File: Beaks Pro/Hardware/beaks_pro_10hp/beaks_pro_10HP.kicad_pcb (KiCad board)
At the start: 2 copper layers, 135.8 x 108.6 mm, 124 parts, among them J1 Pins_02x10_P2.54mm_TH, J11 out1, J12 out2, J13 Eurorack Power, J14 Pins_02x10_P2.54mm_TH, J2 Pins_02x10_P2.54mm_TH, J3 CV1, J4 CV2, J5 CV3, J6 CV4, J7 in1, J8 in2, J9 Pins_02x10_P2.54mm_TH, Q1 2N3904, Q2 2N3904, SW2 SW_Dual, SW3 SW_Mode, SW5 SW_ML6, SW6 SW_ML6, U1 TL072CP, U2 MCP6002-I-P, U3 TL072CP, U4 MCP6002-I-P, U5 TL074, U6 LM4040LP-10, U7 L78L05_TO92, U8 Bluepill, U9 TL072CP

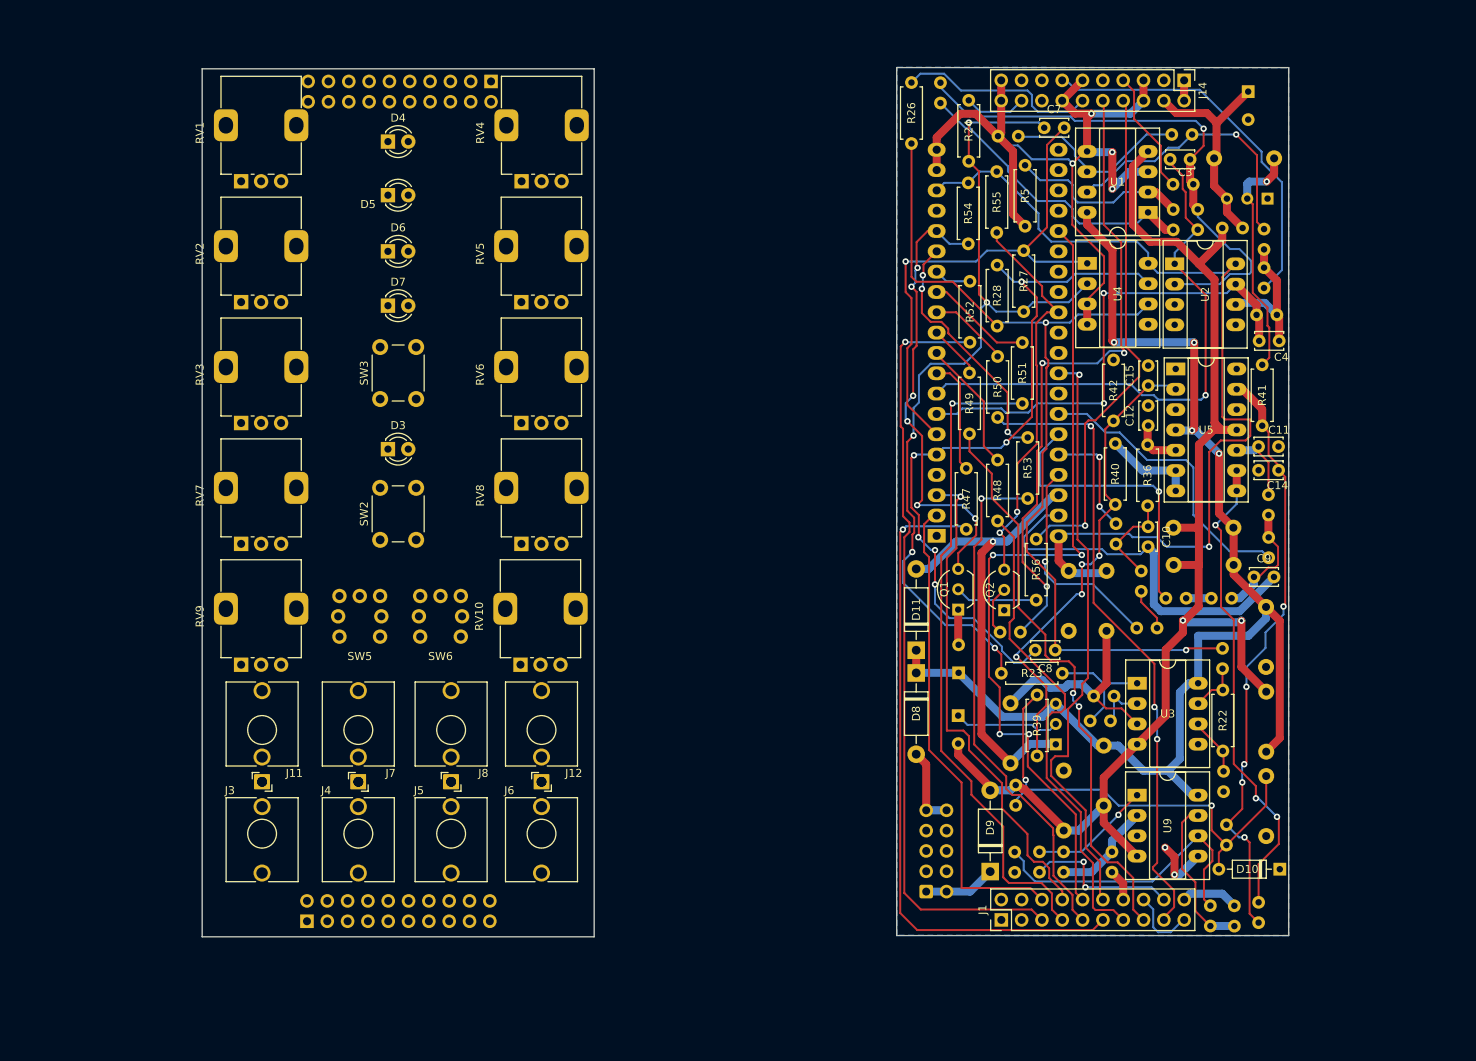
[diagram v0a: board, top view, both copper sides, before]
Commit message: V0.1 Alpha
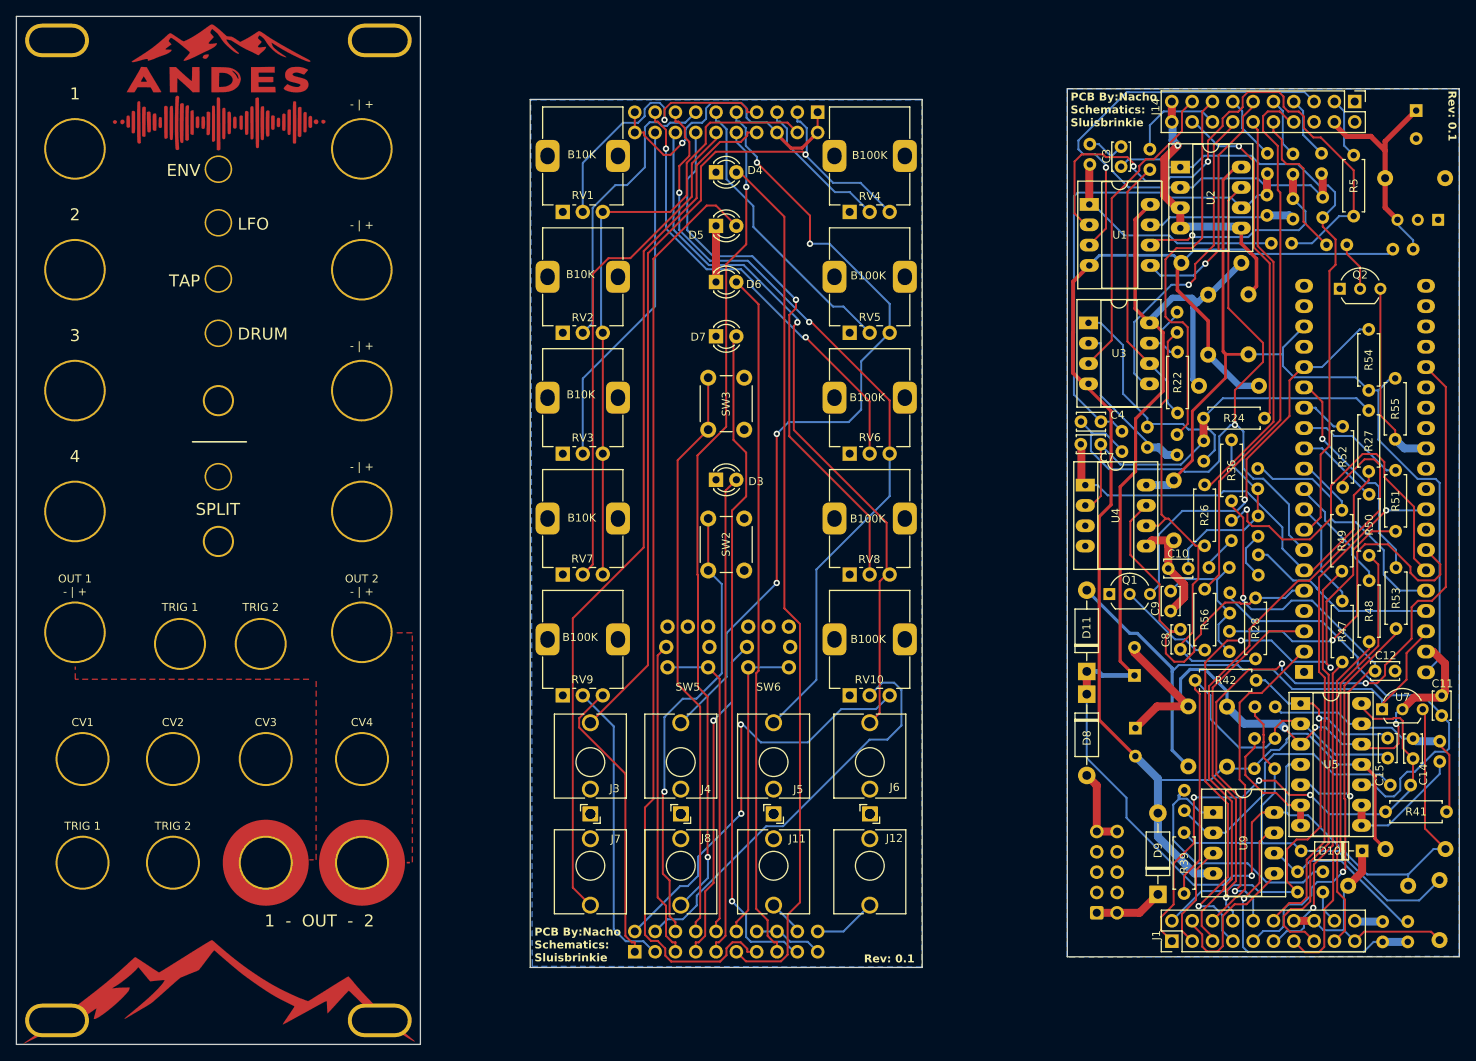
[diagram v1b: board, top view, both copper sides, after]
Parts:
- added ?: , , F.Cu at (70.7, 110.4)
- added ?: , , F.Cu at (93.4, 48.5)
- added ?: , , F.Cu at (57.5, 63.7)
- added ?: , , F.Cu at (75.5, 80.0)
- added ?: , , F.Cu at (69.8, 124.8)
- added ?: , , F.Cu at (57.5, 93.9)
- added ?: , , F.Cu at (57.5, 48.5)
- added ?: , , F.Cu at (93.4, 93.9)
- added ?: , , F.Cu at (69.8, 137.8)
- added ?: , , F.Cu at (58.5, 137.8)
- added ?: , , F.Cu at (93.4, 63.7)
- added ?: , , F.Cu at (93.4, 137.8)
- added ?: , , F.Cu at (57.5, 109.0)
- added ?: , , F.Cu at (57.5, 78.8)
- added ?: , , F.Cu at (75.5, 64.8)
- added ?: , , F.Cu at (75.5, 51.1)
- added ?: , , F.Cu at (75.5, 71.6)
- added ?: , , F.Cu at (93.4, 78.8)
- added ?: , , F.Cu at (81.4, 124.8)
- added ?: , , F.Cu at (80.8, 110.4)
- added ?: , , F.Cu at (81.4, 137.8)
- added ?: , , F.Cu at (75.5, 89.5)
- added ?: , , F.Cu at (93.4, 124.8)
- added ?: , , F.Cu at (58.5, 124.8)
- added ?: , , F.Cu at (75.5, 57.8)
- added ?: , , F.Cu at (75.5, 97.6)
- added ?: , , F.Cu at (93.4, 109.0)
- added REF**: MountingHole_3.2mm_M3, MountingHole:MountingHole_3.2mm_M3, F.Cu at (55.3, 157.5)
- added REF**: MountingHole_3.2mm_M3, MountingHole:MountingHole_3.2mm_M3, F.Cu at (95.6, 157.5)
- added REF**: MountingHole_3.2mm_M3, MountingHole:MountingHole_3.2mm_M3, F.Cu at (55.3, 35.0)
- added REF**: MountingHole_3.2mm_M3, MountingHole:MountingHole_3.2mm_M3, F.Cu at (95.6, 35.0)
- added Ref**: Val**, SVG FRONT PLATE:drawing, F.Cu at (75.2, 40.8)
- added Ref**: Val**, SVG FRONT PLATE:mountains, F.Cu at (75.5, 153.4)
- R23, R40: footprint Resistor_THT:R_Axial_DIN0207_L6.3mm_D2.5mm_P7.62mm_Horizontal -> Resistor_THT:R_Axial_DIN0207_L6.3mm_D2.5mm_P2.54mm_Vertical; moved to B.Cu
- U7: moved to F.Cu
- moved R20 80.8 mm to (191.9, 48.6), turned to -90 degrees
- moved J11 64.1 mm to (144.9, 131.7), turned to 0 degrees
- moved C5 62.7 mm to (203.3, 62.8), turned to 180 degrees
- moved R26 62.2 mm to (198.7, 90.5)
- moved R57 61.7 mm to (214.0, 60.5), turned to 0 degrees
- moved Q2 58.1 mm to (215.6, 66.0), turned to 0 degrees
- moved R41 58.0 mm to (221.4, 131.4), turned to 0 degrees
- moved R54 56.4 mm to (219.3, 78.7), turned to 90 degrees
- moved R55 56.1 mm to (222.6, 77.2)
- moved C15 55.4 mm to (221.6, 124.7)
- moved R24 54.3 mm to (206.2, 82.2), turned to 180 degrees
- moved R28 52.7 mm to (205.1, 112.3)
- moved R52 50.0 mm to (216.0, 90.9)
- moved R47 49.8 mm to (216.0, 112.7)
- moved R49 49.6 mm to (215.9, 101.3)
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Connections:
- C14 pad 2: GND -> /PRE_ATV_OUT1
- C15 pad 2: GND -> /PRE_ATV_OUT2
- J1 pad 1: GND -> /PRE_ATV_OUT1
- J1 pad 2: GND -> /PRE_ATV_OUT2
- J1 pad 3: GND -> /OUT1_ATVPOT
- J1 pad 4: GND -> /OUT2_ATVPOT
- J14 pad 11: GND -> /CV2_ATVPOT
- J14 pad 14: GND -> /CV4_ATVPOT
- J14 pad 15: GND -> /CV3_JACK
- J14 pad 16: GND -> /CV4_JACK
- J14 pad 17: GND -> /CV3_ATVPOT
- J14 pad 3: GND -> /CV1_JACK
- J14 pad 5: GND -> /CV1_ATVPOT
- J14 pad 9: GND -> /CV2_JACK
- J2 pad 1: GND -> GND1
- J2 pad 19: GND -> GND1
- J2 pad 2: GND -> GND1
- J2 pad 20: GND -> GND1
- J2 pad 6: GND -> GND1
- J9 pad 14: GND -> GND1
- J9 pad 16: GND -> GND1
- J9 pad 19: GND -> GND1
- R19 pad 1: GND -> /CV3_JACK
- R20 pad 1: GND -> /CV4_JACK
- R41 pad 1: GND -> /PRE_ATV_OUT1
- R42 pad 1: GND -> /PRE_ATV_OUT2
- R5 pad 1: GND -> /CV1_JACK
- R6 pad 1: GND -> /CV2_JACK
- R60 pad 1: GND -> /PRE_ATV_OUT2
- R64 pad 1: GND -> /PRE_ATV_OUT1
- U1 pad 3: GND -> /CV1_ATVPOT
- U1 pad 5: GND -> /CV2_ATVPOT
- U3 pad 3: GND -> /CV3_ATVPOT
- U3 pad 5: GND -> /CV4_ATVPOT
- U5 pad 1: GND -> /PRE_ATV_OUT2
- U5 pad 14: GND -> /PRE_ATV_OUT1
- U9 pad 3: GND -> /OUT1_ATVPOT
- U9 pad 5: GND -> /OUT2_ATVPOT
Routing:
- net /Front PCB/LED3: track 0.00 -> 117.2 mm
- net /Front PCB/LED2: track 0.00 -> 109.2 mm
- net /Front PCB/TRIG_1: track 0.00 -> 109.2 mm
- net /Front PCB/CV1_JACK: track 0.00 -> 108.9 mm, vias 0 -> 1
- net /Front PCB/TRIG_2: track 0.00 -> 101.6 mm, vias 0 -> 2
- net /Front PCB/CV2_JACK: track 0.00 -> 101.1 mm, vias 0 -> 4
- net /Front PCB/CV3_JACK: track 0.00 -> 97.6 mm, vias 0 -> 2
- net GND: track 252.6 -> 155.2 mm, vias 7 -> 4
- net /Front PCB/CV4_JACK: track 0.00 -> 89.1 mm, vias 0 -> 1
- net /Front PCB/LED4: track 0.00 -> 86.3 mm
- net /Front PCB/LED5: track 0.00 -> 84.5 mm, vias 0 -> 1
- net /Front PCB/-10V_REF: track 0.00 -> 78.6 mm
- net /Front PCB/SW_MODE: track 0.00 -> 72.2 mm
- net /Front PCB/CV4_ATVPOT: track 0.00 -> 68.7 mm, vias 0 -> 1
- net /PRE_ATV_OUT1: track 0.00 -> 66.8 mm, vias 0 -> 3
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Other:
- board size 135.8 x 108.6 mm -> 180.4 x 128.5 mm
- board text added: "- | +"
- board text added: "1"
- board text added: "1 - OUT - 2"
- board text added: "2"
- board text added: "3"
- board text added: "4"
- board text added: "B100K"
- board text added: "B10K"
- board text added: "CV1"
- board text added: "CV2"
- board text added: "CV3"
- board text added: "CV4"
- board text added: "DRUM"
- board text added: "ENV"
- board text added: "LFO"
- board text added: "OUT 1 - | +"
- board text added: "OUT 2 - | +"
- board text added: "PCB By:Nacho Schematics: Sluisbrinkie"
- board text added: "Rev: 0.1"
- board text added: "SPLIT"
- board text added: "TAP"
- board text added: "TRIG 1"
- board text added: "TRIG 2"
- board text added: "USB"
